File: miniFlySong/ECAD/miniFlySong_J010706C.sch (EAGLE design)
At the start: 20 parts, among them J1 BNC, J2 Battery Jack, M1 TEENSY_3.1-3.2_OUTER_ROW, P100 CON14ST2X7_PLUG, T1 PIN2F061.200, T2 PIN2F061.200, U1 MAX931, U2 74AUC1G17DBV, U3 TLP241A(TP1,F, U4 TLP241A(TP1,F

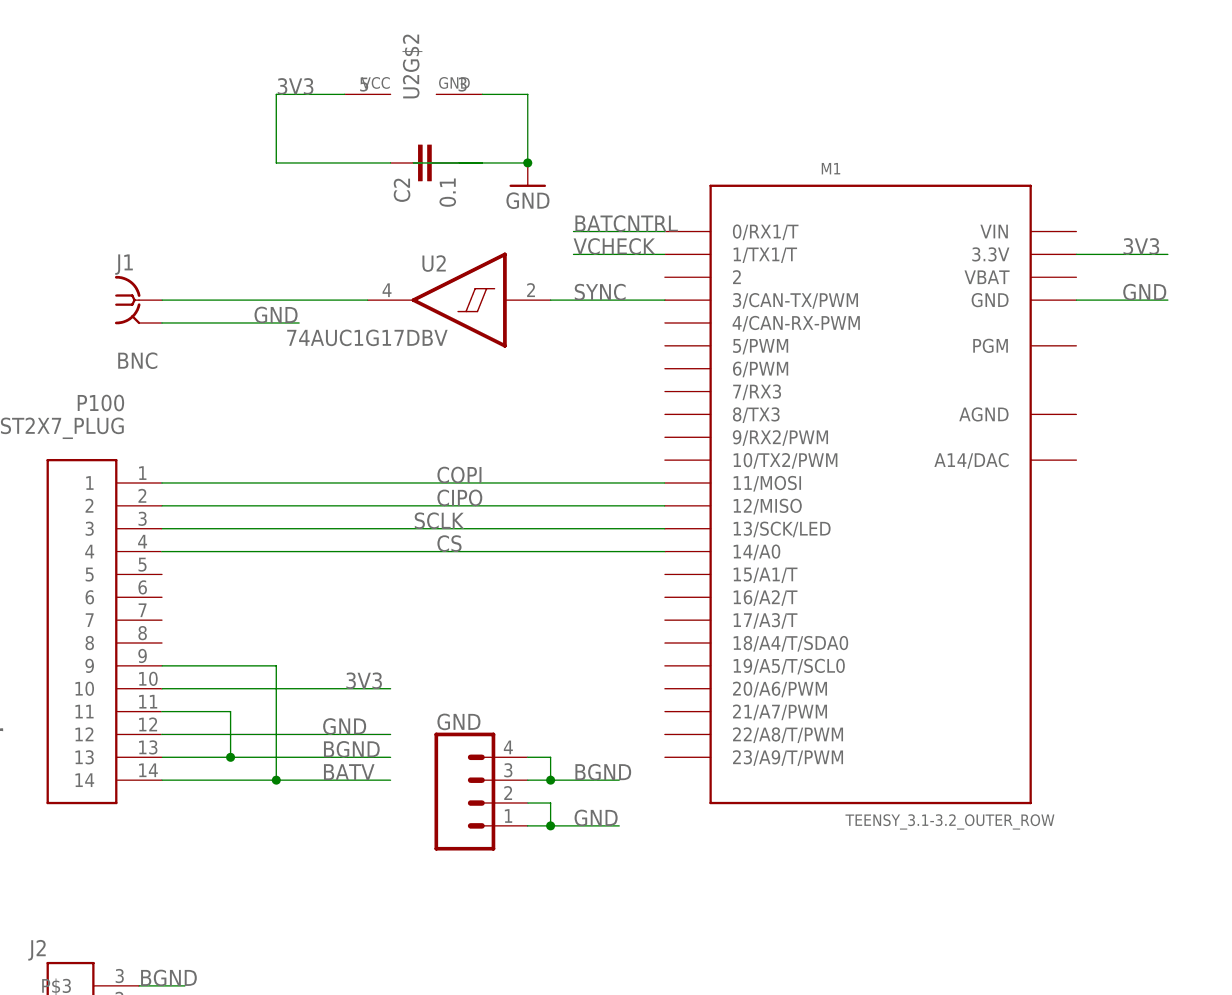
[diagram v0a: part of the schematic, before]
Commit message: Update BOMs and boards, add miniFlySong photo
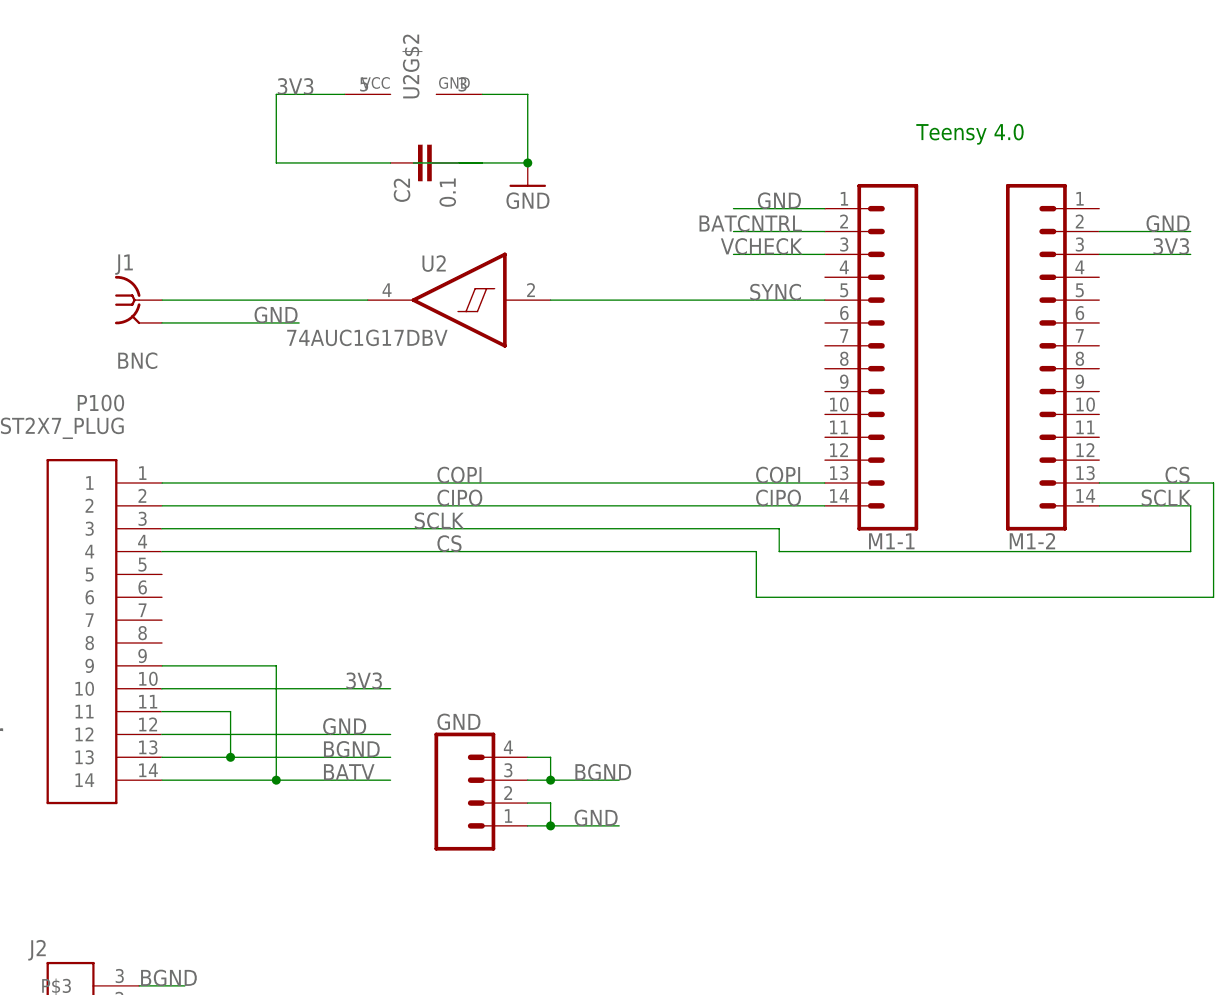
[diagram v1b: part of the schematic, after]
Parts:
- removed M1: TEENSY_3.1-3.2_OUTER_ROW, Teensy_3_and_LC_Series_Boards_v1.4:TEENSY_3.1-3.2_OUTER_ROW
- added M1-1, M1-2: (no value), SparkFun-Connectors:CONN_14
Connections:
- net 3V3: now also M1-2.3; no longer M1.3.3V
- net BATCNTRL: now also M1-1.2; no longer M1.0/RX1/T
- net CIPO: now also M1-1.14; no longer M1.12/MISO
- net COPI: now also M1-1.13; no longer M1.11/MOSI
- net CS: now also M1-2.13; no longer M1.14/A0
- net GND: now also M1-1.1, M1-2.2; no longer M1.GND
- net SCLK: now also M1-2.14; no longer M1.13/SCK/LED
- net SYNC: now also M1-1.5; no longer M1.3/CAN-TX/PWM
- net VCHECK: now also M1-1.3; no longer M1.1/TX1/T
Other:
- note added: "Teensy 4.0"
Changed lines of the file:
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@@
 </classes>
 <parts>
-<part name="M1" library="Teensy_3_and_LC_Series_Boards_v1.4" deviceset="TEENSY_3.1-3.2_OUTER_ROW" device=""/>
 <part name="GND10" library="SparkFun" deviceset="GND" device=""/>
 <part name="C2" library="STEVES_BU" deviceset="CAPS" device="0603S" value="0.1"/>
@@
 <part name="T2" library="con-faston" deviceset="PIN2" device="F061.200"/>
 <part name="T1" library="con-faston" deviceset="PIN2" device="F061.200"/>
+<part name="M1-2" library="SparkFun-Connectors" deviceset="CONN_14" device=""/>
+<part name="M1-1" library="SparkFun-Connectors" deviceset="CONN_14" device=""/>
 </parts>
 <sheets>
@@
    grounds if desired
 </text>
+<text x="58.42" y="81.28" size="1.778" layer="91">Teensy 4.0</text>
 </plain>
 <instances>
-<instance part="M1" gate="G$1" x="53.34" y="43.18"/>
 <instance part="GND10" gate="1" x="15.24" y="76.2" rot="MR0"/>
 <instance part="C2" gate="G$1" x="0" y="78.74" rot="MR270"/>
@@
 <instance part="T2" gate="-1" x="58.42" y="-38.1"/>
 <instance part="T1" gate="-1" x="58.42" y="-48.26"/>
+<instance part="M1-2" gate="G$1" x="68.58" y="55.88" rot="MR180"/>
+<instance part="M1-1" gate="G$1" x="58.42" y="55.88" rot="R180"/>
 </instances>
 <busses>
@@
 <net name="CS" class="0">
 <segment>
-<wire x1="30.48" y1="35.56" x2="-25.4" y2="35.56" width="0.1524" layer="91"/>
+<wire x1="40.64" y1="35.56" x2="-25.4" y2="35.56" width="0.1524" layer="91"/>
 <label x="5.08" y="35.56" size="1.778" layer="95"/>
-<pinref part="M1" gate="G$1" pin="14/A0"/>
 <pinref part="P100" gate="G$1" pin="4"/>
+<wire x1="40.64" y1="35.56" x2="40.64" y2="30.48" width="0.1524" layer="91"/>
+<wire x1="40.64" y1="30.48" x2="91.44" y2="30.48" width="0.1524" layer="91"/>
+<wire x1="91.44" y1="30.48" x2="91.44" y2="43.18" width="0.1524" layer="91"/>
+<pinref part="M1-2" gate="G$1" pin="13"/>
+<wire x1="78.74" y1="43.18" x2="91.44" y2="43.18" width="0.1524" layer="91"/>
+<label x="88.9" y="43.18" size="1.778" layer="95" rot="MR0"/>
 </segment>
 </net>
 <net name="SCLK" class="0">
 <segment>
-<wire x1="30.48" y1="38.1" x2="-25.4" y2="38.1" width="0.1524" layer="91"/>
+<wire x1="43.18" y1="38.1" x2="-25.4" y2="38.1" width="0.1524" layer="91"/>
 <label x="2.54" y="38.1" size="1.778" layer="95"/>
-<pinref part="M1" gate="G$1" pin="13/SCK/LED"/>
 <pinref part="P100" gate="G$1" pin="3"/>
+<wire x1="43.18" y1="38.1" x2="43.18" y2="35.56" width="0.1524" layer="91"/>
+<pinref part="M1-2" gate="G$1" pin="14"/>
+<wire x1="78.74" y1="40.64" x2="88.9" y2="40.64" width="0.1524" layer="91"/>
+<label x="88.9" y="40.64" size="1.778" layer="95" rot="MR0"/>
+<wire x1="43.18" y1="35.56" x2="88.9" y2="35.56" width="0.1524" layer="91"/>
+<wire x1="88.9" y1="35.56" x2="88.9" y2="40.64" width="0.1524" layer="91"/>
 </segment>
 </net>
 <net name="CIPO" class="0">
 <segment>
-<wire x1="30.48" y1="40.64" x2="-25.4" y2="40.64" width="0.1524" layer="91"/>
+<pinref part="M1-1" gate="G$1" pin="14"/>
+<label x="45.72" y="40.64" size="1.778" layer="95" rot="MR0"/>
+<wire x1="48.26" y1="40.64" x2="-25.4" y2="40.64" width="0.1524" layer="91"/>
 <label x="5.08" y="40.64" size="1.778" layer="95"/>
-<pinref part="M1" gate="G$1" pin="12/MISO"/>
 <pinref part="P100" gate="G$1" pin="2"/>
 </segment>
@@
 <net name="COPI" class="0">
 <segment>
-<wire x1="30.48" y1="43.18" x2="-25.4" y2="43.18" width="0.1524" layer="91"/>
+<pinref part="M1-1" gate="G$1" pin="13"/>
+<label x="45.72" y="43.18" size="1.778" layer="95" rot="MR0"/>
+<wire x1="48.26" y1="43.18" x2="-25.4" y2="43.18" width="0.1524" layer="91"/>
 <label x="5.08" y="43.18" size="1.778" layer="95"/>
-<pinref part="M1" gate="G$1" pin="11/MOSI"/>
 <pinref part="P100" gate="G$1" pin="1"/>
 </segment>
 </net>
 <net name="GND" class="0">
-<segment>
-<wire x1="76.2" y1="63.5" x2="86.36" y2="63.5" width="0.1524" layer="91"/>
-<label x="81.28" y="63.5" size="1.778" layer="95"/>
-<pinref part="M1" gate="G$1" pin="GND"/>
-</segment>
 <segment>
 <wire x1="-25.4" y1="15.24" x2="0" y2="15.24" width="0.1524" layer="91"/>
@@
 <label x="12.7" y="-27.94" size="1.778" layer="95"/>
 </segment>
+<segment>
+<pinref part="M1-1" gate="G$1" pin="1"/>
+<wire x1="48.26" y1="73.66" x2="38.1" y2="73.66" width="0.1524" layer="91"/>
+<label x="45.72" y="73.66" size="1.778" layer="95" rot="MR0"/>
+</segment>
+<segment>
+<pinref part="M1-2" gate="G$1" pin="2"/>
+<wire x1="78.74" y1="71.12" x2="88.9" y2="71.12" width="0.1524" layer="91"/>
+<label x="88.9" y="71.12" size="1.778" layer="95" rot="MR0"/>
+</segment>
 </net>
 <net name="BAT+" class="0">
@@
 <label x="-5.08" y="20.32" size="1.778" layer="95"/>
 <pinref part="P100" gate="G$1" pin="10"/>
-</segment>
-<segment>
-<pinref part="M1" gate="G$1" pin="3.3V"/>
-<wire x1="76.2" y1="68.58" x2="86.36" y2="68.58" width="0.1524" layer="91"/>
-<label x="81.28" y="68.58" size="1.778" layer="95"/>
 </segment>
 <segment>
@@
 <label x="-12.7" y="86.36" size="1.778" layer="95"/>
 </segment>
+<segment>
+<pinref part="M1-2" gate="G$1" pin="3"/>
+<wire x1="78.74" y1="68.58" x2="88.9" y2="68.58" width="0.1524" layer="91"/>
+<label x="88.9" y="68.58" size="1.778" layer="95" rot="MR0"/>
+</segment>
 </net>
 <net name="SYNC" class="0">
 <segment>
-<pinref part="M1" gate="G$1" pin="3/CAN-TX/PWM"/>
+<pinref part="M1-1" gate="G$1" pin="5"/>
+<label x="45.72" y="63.5" size="1.778" layer="95" rot="MR0"/>
 <pinref part="U2" gate="G$1" pin="I"/>
-<wire x1="30.48" y1="63.5" x2="17.78" y2="63.5" width="0.1524" layer="91"/>
-<label x="20.32" y="63.5" size="1.778" layer="95"/>
+<wire x1="48.26" y1="63.5" x2="17.78" y2="63.5" width="0.1524" layer="91"/>
 </segment>
 </net>
@@
 <net name="VCHECK" class="0">
 <segment>
-<pinref part="M1" gate="G$1" pin="1/TX1/T"/>
-<wire x1="30.48" y1="68.58" x2="20.32" y2="68.58" width="0.1524" layer="91"/>
-<label x="20.32" y="68.58" size="1.778" layer="95"/>
+<pinref part="M1-1" gate="G$1" pin="3"/>
+<wire x1="48.26" y1="68.58" x2="38.1" y2="68.58" width="0.1524" layer="91"/>
+<label x="45.72" y="68.58" size="1.778" layer="95" rot="MR0"/>
 </segment>
 </net>
@@
 <net name="BATCNTRL" class="0">
 <segment>
-<pinref part="M1" gate="G$1" pin="0/RX1/T"/>
-<wire x1="30.48" y1="71.12" x2="20.32" y2="71.12" width="0.1524" layer="91"/>
-<label x="20.32" y="71.12" size="1.778" layer="95"/>
-</segment>
-<segment>
 <pinref part="R7" gate="G$1" pin="1"/>
 <wire x1="35.56" y1="-17.78" x2="40.64" y2="-17.78" width="0.1524" layer="91"/>
 <label x="38.1" y="-17.78" size="1.778" layer="95"/>
 </segment>
-</net>
+<segment>
+<pinref part="M1-1" gate="G$1" pin="2"/>
+<wire x1="48.26" y1="71.12" x2="38.1" y2="71.12" width="0.1524" layer="91"/>
+<label x="45.72" y="71.12" size="1.778" layer="95" rot="MR0"/>
+</segment>
+</net>
